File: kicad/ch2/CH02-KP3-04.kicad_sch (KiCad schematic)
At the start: 7 parts

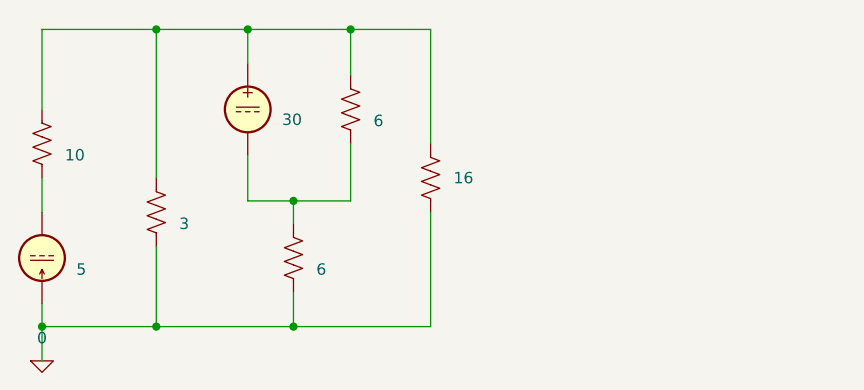
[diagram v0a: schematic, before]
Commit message: regular
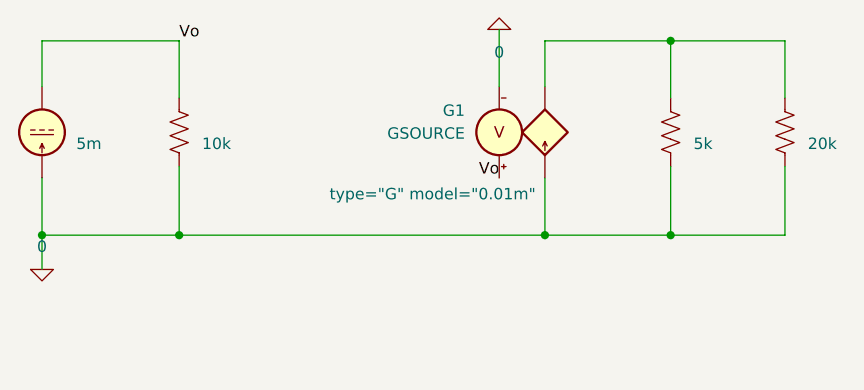
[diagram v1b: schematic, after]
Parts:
- removed I6: 5, symbol Simulation_SPICE:IDC
- removed R29: 10, symbol Device:R_US
- removed R30: 3, symbol Device:R_US
- removed R31, R32: 6, symbol Device:R_US
- removed R33: 16, symbol Device:R_US
- removed V12: 30, symbol Simulation_SPICE:VDC
- added G1: GSOURCE, symbol Simulation_SPICE:GSOURCE
- added I7: 5m, symbol Simulation_SPICE:IDC
- added R34: 10k, symbol Device:R_US
- added R35: 5k, symbol Device:R_US
- added R36: 20k, symbol Device:R_US
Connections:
- net 0: now also G1.1 (N+), G1.4 (C-), I7.1, R34.2, R35.2, R36.2
- new net: G1.2 (N-), R35.1, R36.1
- new net Vo: G1.3 (C+), I7.2, R34.1
